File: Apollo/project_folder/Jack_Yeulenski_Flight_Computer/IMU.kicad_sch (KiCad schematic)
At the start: 3 parts, among them U1 BMI088

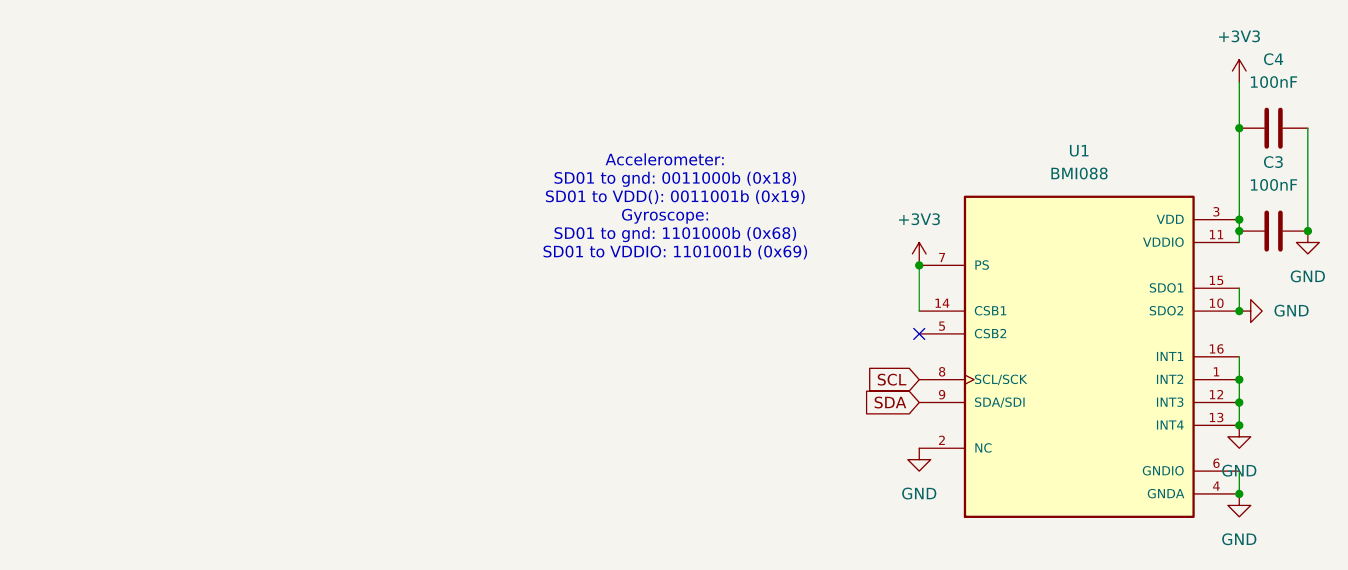
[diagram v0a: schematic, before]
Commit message: Revert "Merge branch 'main' of https://github.com/Terrapin-Rocket-Team/SRAD-Avionics"
This reverts commit e5f68e4e525f2a5ad7eebbc917cc2807b67ca5e1, reversing
changes made to 8a40e2e341d8980ca528983581171a8bd9cc0146.
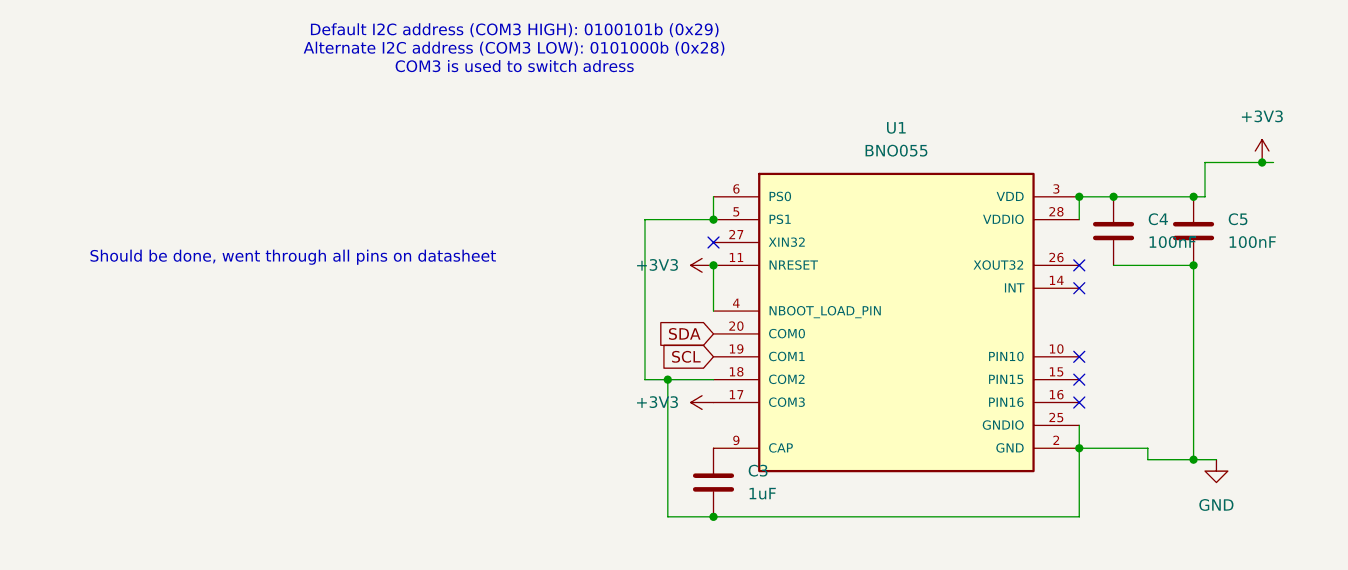
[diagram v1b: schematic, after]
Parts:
- removed U1: BMI088, BMI088 (1):PQFN50P450X300X100-16N, symbol BMI088:BMI088
- added C5: 100nF, Capacitor_SMD:C_0805_2012Metric, symbol Device:C
- added U1: BNO055, Package_LGA:LGA-28_5.2x3.8mm_P0.5mm, symbol SRAD:BNO055
- C3: value 100nF -> 1uF; footprint Capacitor_SMD:C_0603_1608Metric -> Capacitor_SMD:C_0805_2012Metric
- C4: footprint Capacitor_SMD:C_0603_1608Metric -> Capacitor_SMD:C_0805_2012Metric
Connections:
- net +3V3: now also C5.1, U1.11 (NRESET), U1.17 (COM3), U1.28 (VDDIO), U1.3 (VDD), U1.4 (NBOOT_LOAD_PIN); no longer C3.1
- net GND: now also C3.1, C5.2, U1.18 (COM2), U1.2 (GND), U1.25 (GNDIO), U1.5 (PS1), U1.6 (PS0); no longer C3.2
- net SCL: now also U1.19 (COM1)
- net SDA: now also U1.20 (COM0)
- new net: C3.2, U1.9 (CAP)
- no-connect marks 1 -> 6
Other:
- note added: "Default I2C address (COM3 HIGH): 0100101b (0x29) Alternate I2C address (COM3 LOW): 0101000b (0x28) COM3 is used to switch adress"
- note added: "Should be done, went through all pins on datasheet"
- note removed: "Accelerometer: SD01 to gnd: 0011000b (0x18) SD01 to VDD(): 0011001b (0x19) Gyroscope: SD01 to gnd: 1101000b (0x68) SD01 to VDDIO: 1101001b (0x69)"
